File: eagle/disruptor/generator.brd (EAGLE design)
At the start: 127 x 76.2 mm, 29 parts, among them IC1 NE555, IC2 74ALS04N, IC3 IR2110, IC4 7805TV, J1 PIN2F061.100, J2 PIN2F061.100, J3 PIN2F061.100, J4 PIN2F061.100, J5 PIN2F061.100, J6 PIN2F061.100, Q1 STP11NM60, Q2 STP11NM60

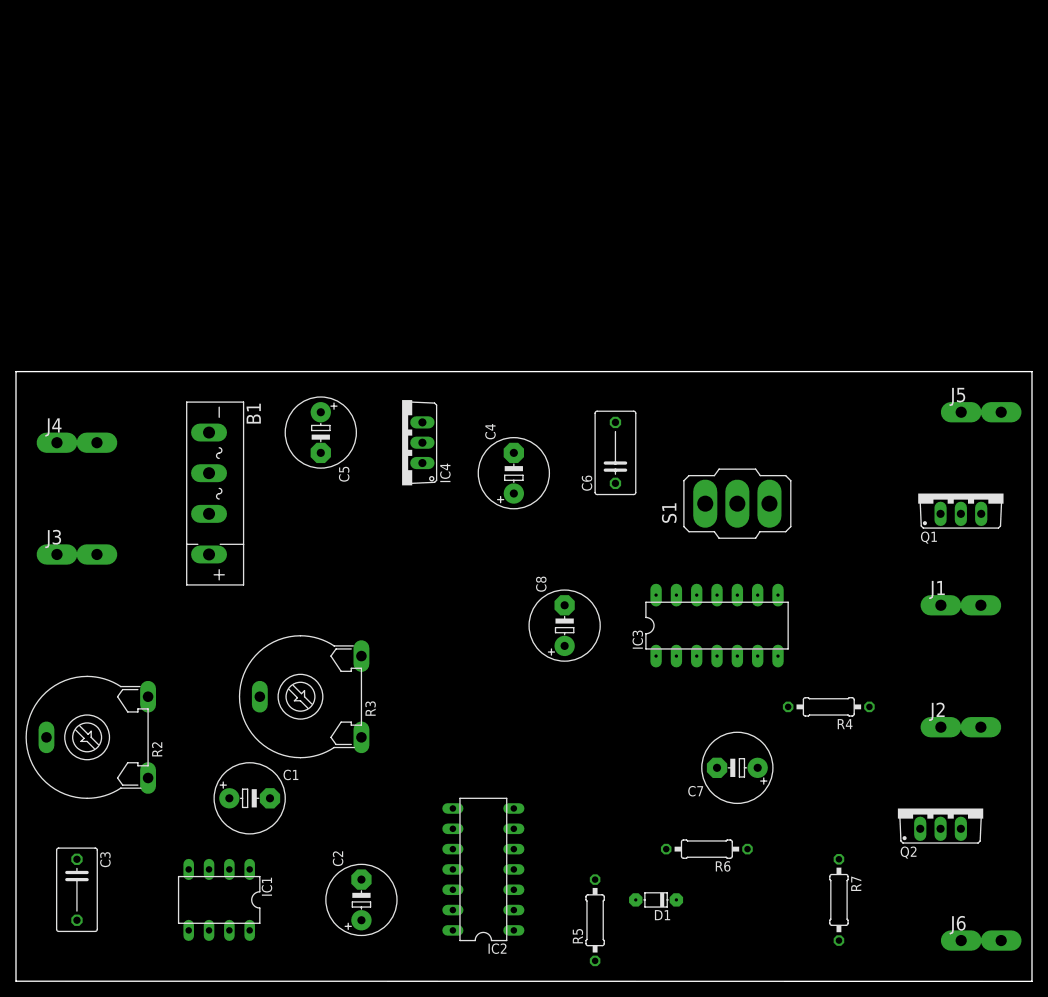
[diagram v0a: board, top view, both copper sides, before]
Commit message: layouts
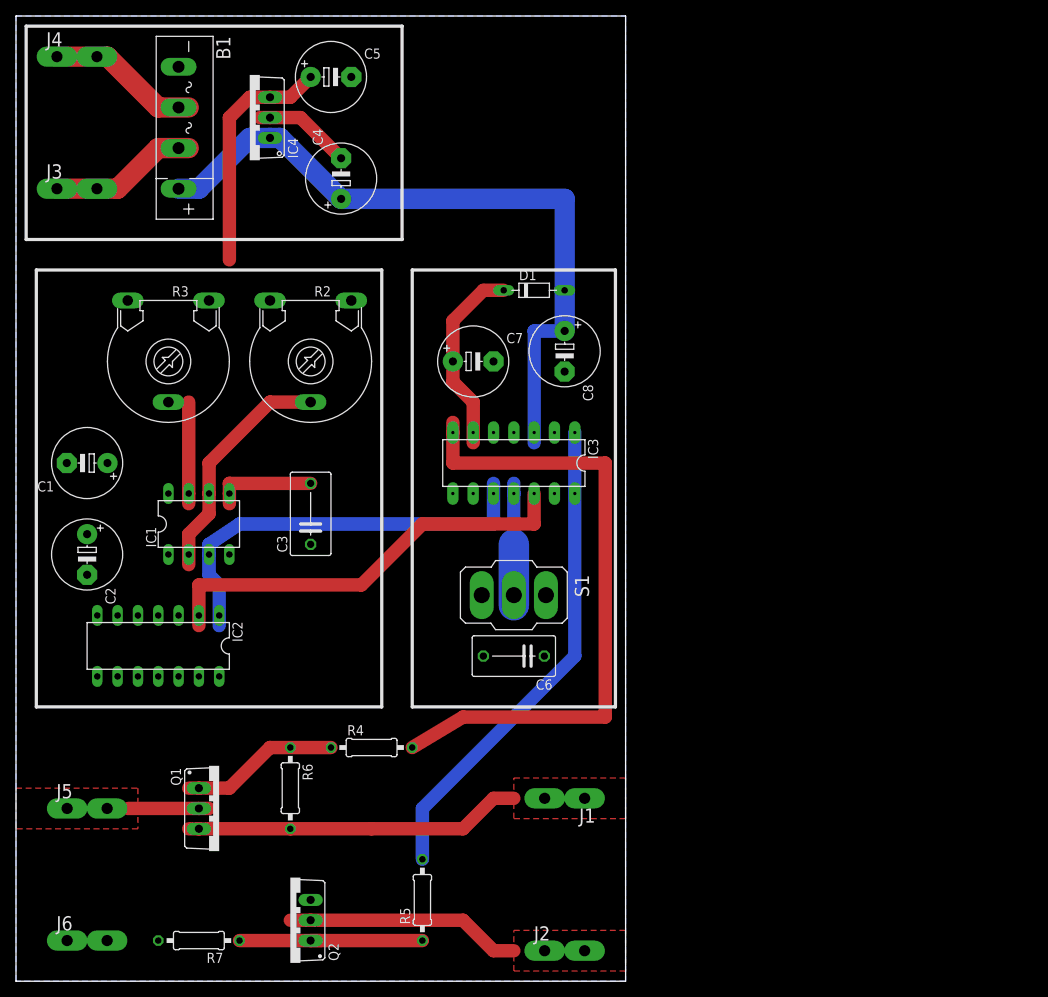
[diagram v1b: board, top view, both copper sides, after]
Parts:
- D1: device diode:D-5 -> diode:D-7.5
- moved J5 122.2 mm to (8.89, 21.6)
- moved J6 111.8 mm to (8.89, 5.08)
- moved Q1 100.7 mm to (25.4, 21.6), turned to 270 degrees
- moved Q2 82.5 mm to (34.3, 7.62), turned to 90 degrees
- moved R7 80.2 mm to (22.9, 5.08), turned to 180 degrees
- moved D1 77.7 mm to (64.8, 86.4), turned to 0 degrees
- moved C7 60.6 mm to (57.1, 77.5), turned to 0 degrees
- moved R4 57.4 mm to (44.5, 29.2), turned to 0 degrees
- moved J2 56.9 mm to (68.6, 3.81)
- moved C3 55.3 mm to (36.8, 58.4), turned to 90 degrees
- moved C2 55.1 mm to (8.89, 53.3), turned to 270 degrees
- moved J1 55.1 mm to (68.6, 22.9), turned to 180 degrees
- moved R2 54.7 mm to (36.8, 77.5), turned to 180 degrees
- moved R6 52.6 mm to (34.3, 24.1), turned to 270 degrees
- moved IC2 49.3 mm to (17.8, 41.9), turned to 180 degrees
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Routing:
- net VDD: track 0.00 -> 88.3 mm
- net HO: track 0.00 -> 81.1 mm
- net LO: track 0.00 -> 61.2 mm
- net LIN: track 0.00 -> 54.0 mm
- net HIN: track 0.00 -> 52.1 mm
- net TRANS1: track 0.00 -> 42.2 mm
- net VCC: track 0.00 -> 30.0 mm
- net N$2: track 0.00 -> 29.6 mm
- net TRANS2: track 0.00 -> 29.5 mm
- net N$1: track 0.00 -> 24.2 mm
- net N$11: track 0.00 -> 24.1 mm
- net N$12: track 0.00 -> 19.9 mm
- net N$9: track 0.00 -> 19.1 mm
- net N$10: track 0.00 -> 18.6 mm
- net N$17: track 0.00 -> 15.2 mm
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- added copper zone on layer 16, net GND
- added copper zone on layer 1, net N$13
- added copper zone on layer 1, net TRANS1
- added copper zone on layer 1, net TRANS2
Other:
- board size 127 x 76.2 mm -> 76.2 x 120.7 mm
